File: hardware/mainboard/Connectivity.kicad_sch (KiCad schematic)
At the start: 38 parts, among them U12 LM393, U13 LM393, U14 LM393, U2 FT230XS, U6 MCP2542FD-E/MF, U7 MCP2542FD-E/MF

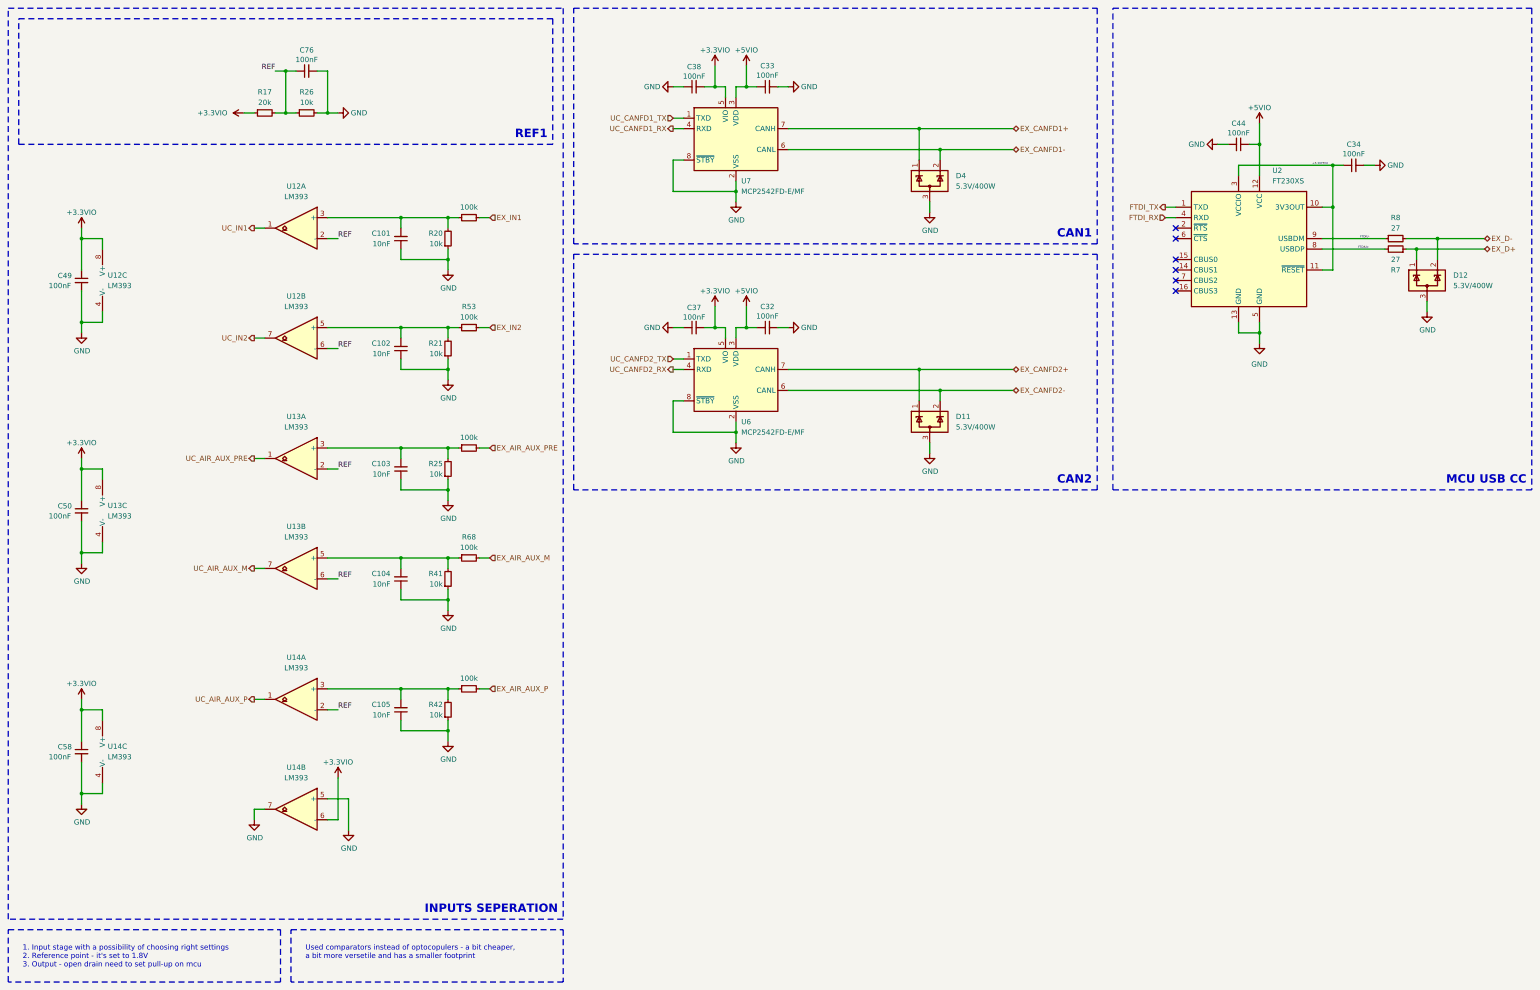
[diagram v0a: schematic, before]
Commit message: isolation with every thing
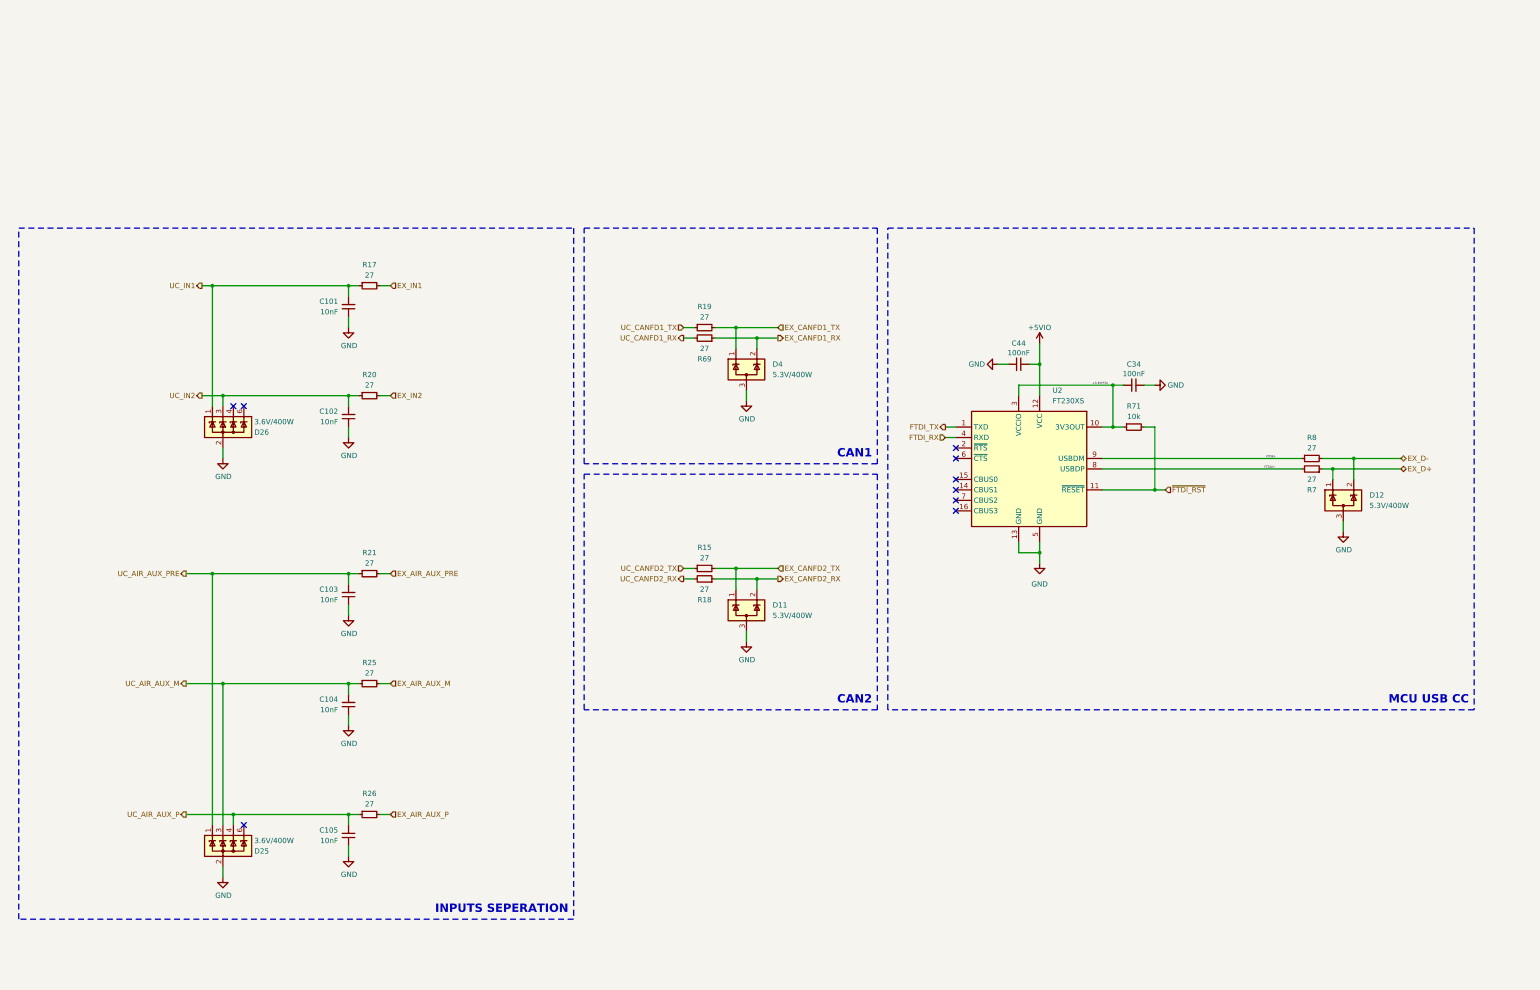
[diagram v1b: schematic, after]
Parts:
- removed C32, C33, C37, C38, C49, C50, C58, C76: 100nF, Capacitor_SMD:C_0603_1608Metric, symbol Device:C_Small
- removed R41, R42: 10k, Resistor_SMD:R_0603_1608Metric, symbol Device:R_Small
- removed R49, R53, R63, R68, R70: 100k, Resistor_SMD:R_0603_1608Metric, symbol Device:R_Small
- removed U12, U13, U14: LM393, Package_SO:VSSOP-8_3x3mm_P0.65mm, symbol Comparator:LM393
- removed U6, U7: MCP2542FD-E/MF, Package_DFN_QFN:DFN-8-1EP_3x3mm_P0.65mm_EP1.55x2.4mm, symbol Interface_CAN_LIN:MCP2542FDxMF
- added D25, D26: 3.6V/400W, Package_TO_SOT_SMD:SOT-23-6, symbol Power_Protection:ESDA5V3SC5
- added R15, R18, R19, R69: 27, Resistor_SMD:R_0603_1608Metric, symbol Device:R_Small
- added R71: 10k, Resistor_SMD:R_0603_1608Metric, symbol Device:R_Small
- R17: value 20k -> 27; Mouser Part Number -- -> 71-CRCW060333R0FKEC
- R20, R21, R25, R26: value 10k -> 27; Mouser Part Number -- -> 71-CRCW060333R0FKEC
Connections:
- net +3.3VIO is gone; now on net UC_IN1: R17.1
- net +3.3VFTDI: now also R71.1; no longer U2.11 (~{RESET})
- net EX_AIR_AUX_M: now also R25.2
- net EX_AIR_AUX_P: now also R26.2
- net EX_AIR_AUX_PRE: now also R21.2
- net EX_IN1: now also R17.2
- net EX_IN2: now also R20.2
- net GND: now also D25.2 (K), D25.5 (NC), D26.2 (K), D26.5 (NC); no longer R20.1, R21.1, R25.1, R26.2
- net UC_AIR_AUX_M: now also C104.2, R25.1, D25.3 (A)
- net UC_AIR_AUX_P: now also C105.2, R26.1, D25.4 (A)
- net UC_AIR_AUX_PRE: now also C103.2, R21.1, D25.1 (A)
- net UC_CANFD1_RX: now also R69.2
- net UC_CANFD1_TX: now also R19.1
- net UC_CANFD2_RX: now also R18.2
- net UC_CANFD2_TX: now also R15.1
- net UC_IN1: now also C101.2, D26.1 (A)
- net UC_IN2: now also C102.2, R20.1, D26.3 (A)
- net EX_CANFD1+ renamed EX_CANFD1_TX
- net EX_CANFD1_TX: now also R19.2
- net EX_CANFD1- renamed EX_CANFD1_RX
- net EX_CANFD1_RX: now also R69.1
- net EX_CANFD2+ renamed EX_CANFD2_TX
- net EX_CANFD2_TX: now also R15.2
- net EX_CANFD2- renamed EX_CANFD2_RX
- net EX_CANFD2_RX: now also R18.1
- removed net REF: R17.2, R26.1
- new net ~{FTDI_RST}: R71.2, U2.11 (~{RESET})
- no-connect marks 6 -> 9
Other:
- note removed: "REF1"
- moved on the sheet: C101, C102, C34, C44, D11, D12, D4, R7, R8, U2
